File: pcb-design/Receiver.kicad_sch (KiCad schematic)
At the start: 29 parts, among them J6 USB_A, J9 ARM_JTAG, SW2 SW_Push, U1 ATmega32A-A, U2 nRF51x22-QFxx, U3 AMS1117-3.3, Y1 16MHz, Y3 16MHz

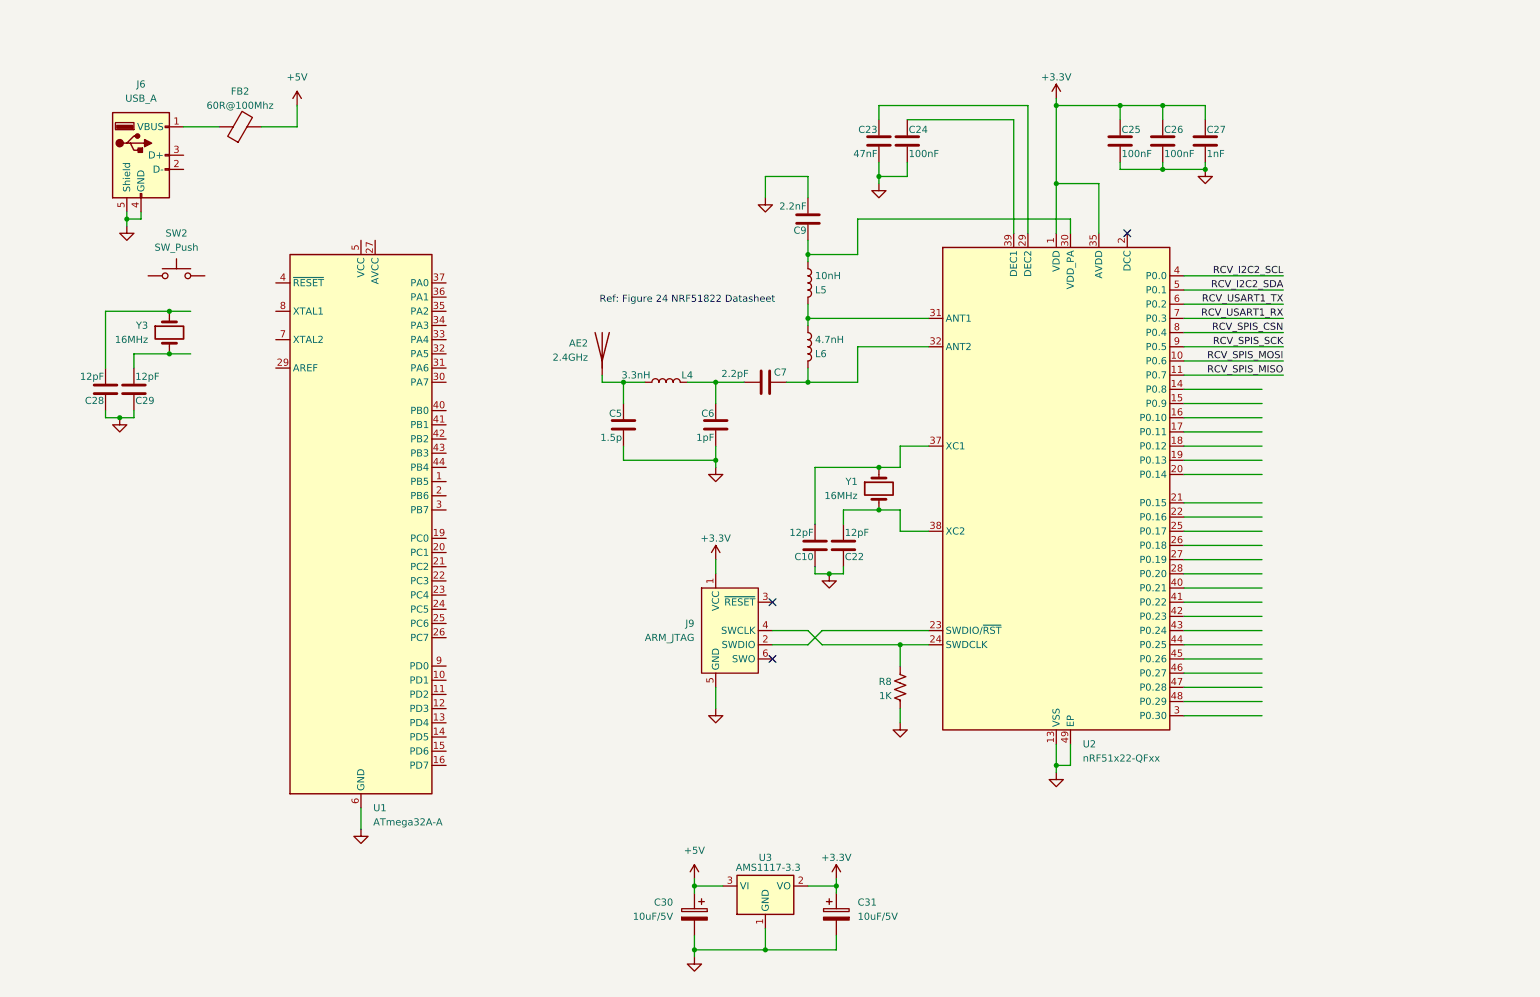
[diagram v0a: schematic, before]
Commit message: [minggu 7 juli 8:55] cleaning schematic layout
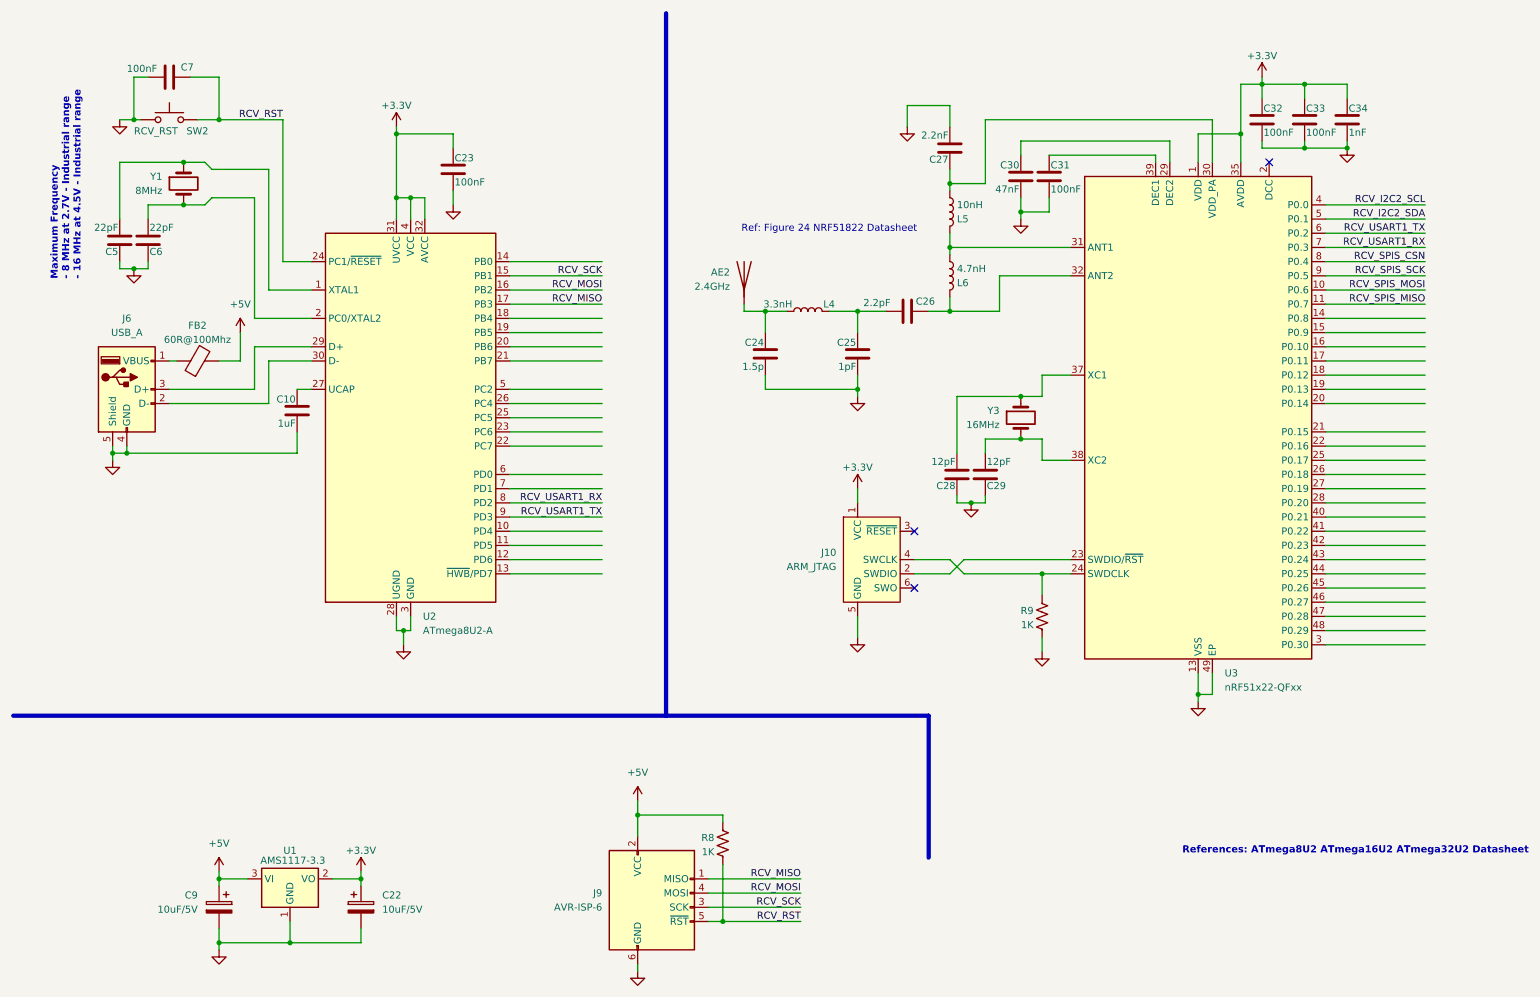
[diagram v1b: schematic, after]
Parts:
- removed U1: ATmega32A-A, Package_QFP:TQFP-44_10x10mm_P0.8mm, symbol MCU_Microchip_ATmega:ATmega32A-A
- added C10: 1uF, symbol Device:C
- added C23, C7: 100nF, symbol Device:C
- added J9: AVR-ISP-6, symbol Connector:AVR-ISP-6
- added R8: 1K, Resistor_SMD:R_1206_3216Metric, symbol Device:R_US
- added U2: ATmega8U2-A, Package_QFP:TQFP-32_7x7mm_P0.8mm, symbol MCU_Microchip_ATmega:ATmega8U2-A
- C5: renamed from C28; value 12pF -> 22pF
- C6: renamed from C29; value 12pF -> 22pF
- SW2: value SW_Push -> RCV_RST
- Y1: renamed from Y3; value 16MHz -> 8MHz
- renumbered C31 to C22, C5 to C24, C6 to C25, C7 to C26, C9 to C27, C10 to C28, C22 to C29, C23 to C30, C24 to C31, C25 to C32, C26 to C33, C27 to C34, C30 to C9, J9 to J10, R8 to R9, U3 to U1, U2 to U3, Y1 to Y3
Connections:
- net +3.3V: now also C23.1, U2.31 (UVCC), U2.32 (AVCC), U2.4 (VCC)
- net +5V: now also J9.2 (VCC), R8.2
- net GND: now also SW2.1, C10.2, C23.2, C7.2, J9.6 (GND), U2.28 (UGND), U2.3 (GND)
- net RCV_USART1_RX: now also U2.8 (PD2)
- net RCV_USART1_TX: now also U2.9 (PD3)
- net at C6.2, Y1.2: now also U2.2 (PC0/XTAL2)
- net at C5.2, Y1.1: now also U2.1 (XTAL1)
- net at J6.2 (D-): now also U2.30 (D-)
- net at J6.3 (D+): now also U2.29 (D+)
- net RCV_RST: now reaches SW2.2
- net RCV_RST: now also C7.1, J9.5 (~{RST}), R8.1, U2.24 (PC1/~{RESET})
- new net: C10.1, U2.27 (UCAP)
- new net RCV_MISO: J9.1 (MISO), U2.17 (PB3)
- new net RCV_MOSI: J9.4 (MOSI), U2.16 (PB2)
- new net RCV_SCK: J9.3 (SCK), U2.15 (PB1)
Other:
- note added: "Maximum Frequency - 8 MHz at 2.7V - Industrial range - 16 MHz at 4.5V - Industrial range"
- note added: "References: ATmega8U2 ATmega16U2 ATmega32U2 Datasheet"
- moved on the sheet: AE2, C22, C24, C25, C26, C27, C28, C29, C30, C31, C32, C33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
